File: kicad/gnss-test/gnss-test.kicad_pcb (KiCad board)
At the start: 2 copper layers, 17.2 x 36.6 mm, 16 parts, among them J1 PWR, J2 EN, J3 UART, Q1 BSS84, Q2 BSS84, U1 MAX-M10M-00B

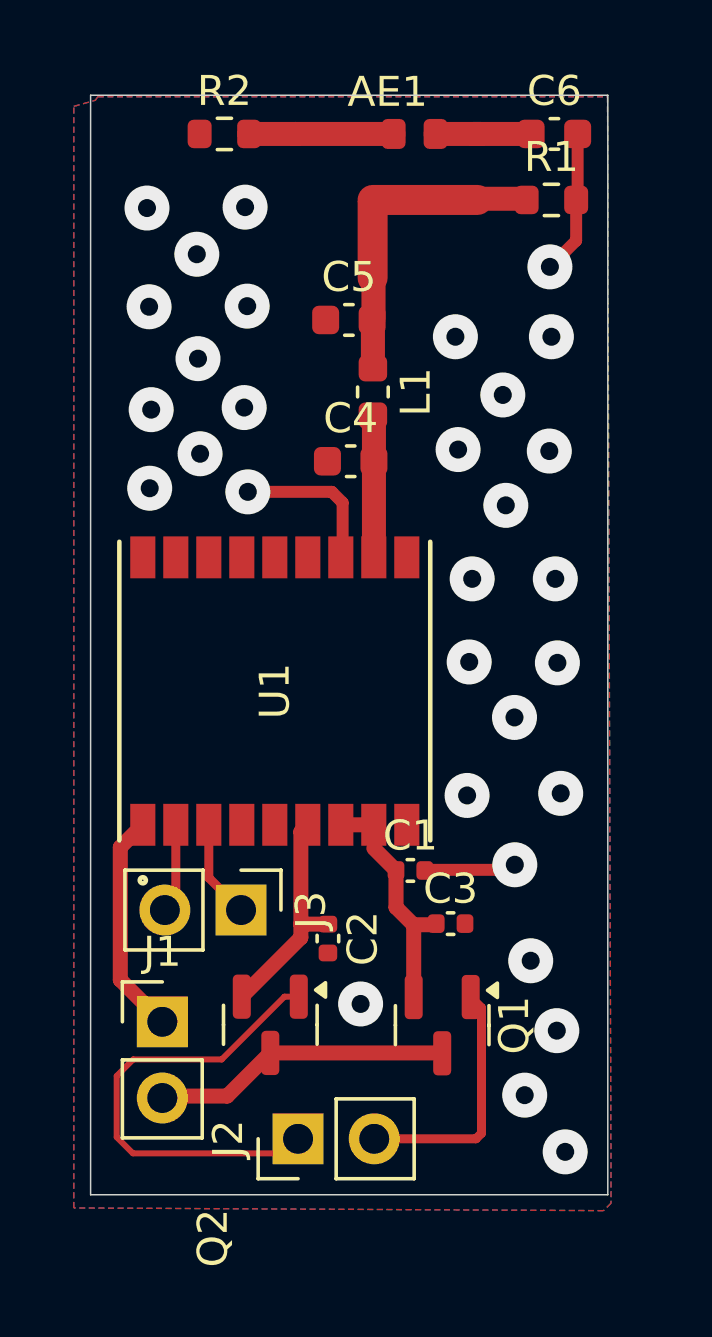
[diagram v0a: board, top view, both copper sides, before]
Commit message: kicad 9.0 updates
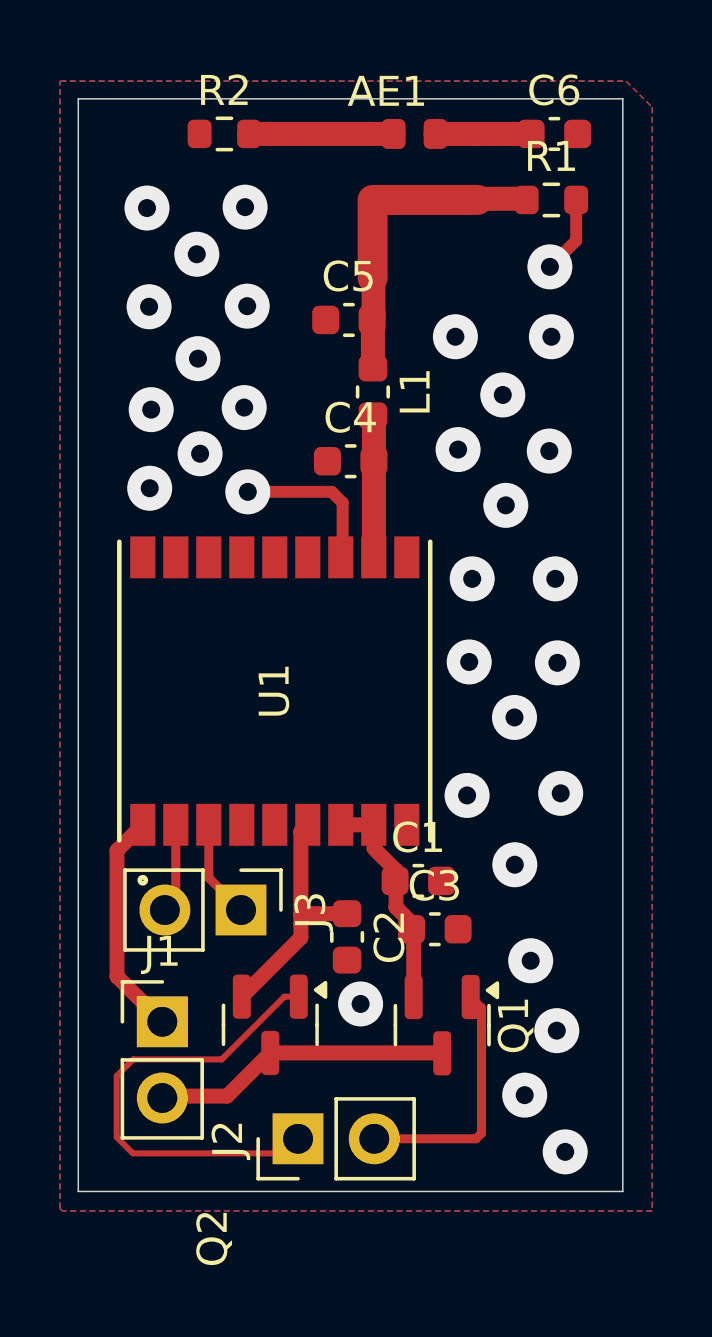
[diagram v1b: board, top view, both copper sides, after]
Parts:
- C1, C2: footprint Capacitor_SMD:C_0402_1005Metric -> Capacitor_SMD:C_0603_1608Metric
- C3: value 100n -> 1u; footprint Capacitor_SMD:C_0402_1005Metric -> Capacitor_SMD:C_0603_1608Metric
- moved C2 0.64 mm to (163.8, 79.1)
- moved C3 0.56 mm to (166.7, 78.8)
- moved C1 0.44 mm to (166.2, 77.2)
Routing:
- net GND: track 21.1 -> 16.2 mm
- net Net-(Q1-S): track 8.18 -> 7.41 mm
- net Net-(Q2-S): track 7.54 -> 8.20 mm
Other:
- board size 17.2 x 36.6 mm -> 18.2 x 36.4 mm
